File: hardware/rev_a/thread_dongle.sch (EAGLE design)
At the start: 5 parts, among them IC1 CP2102, J1 USB-A-MALE-PLUG

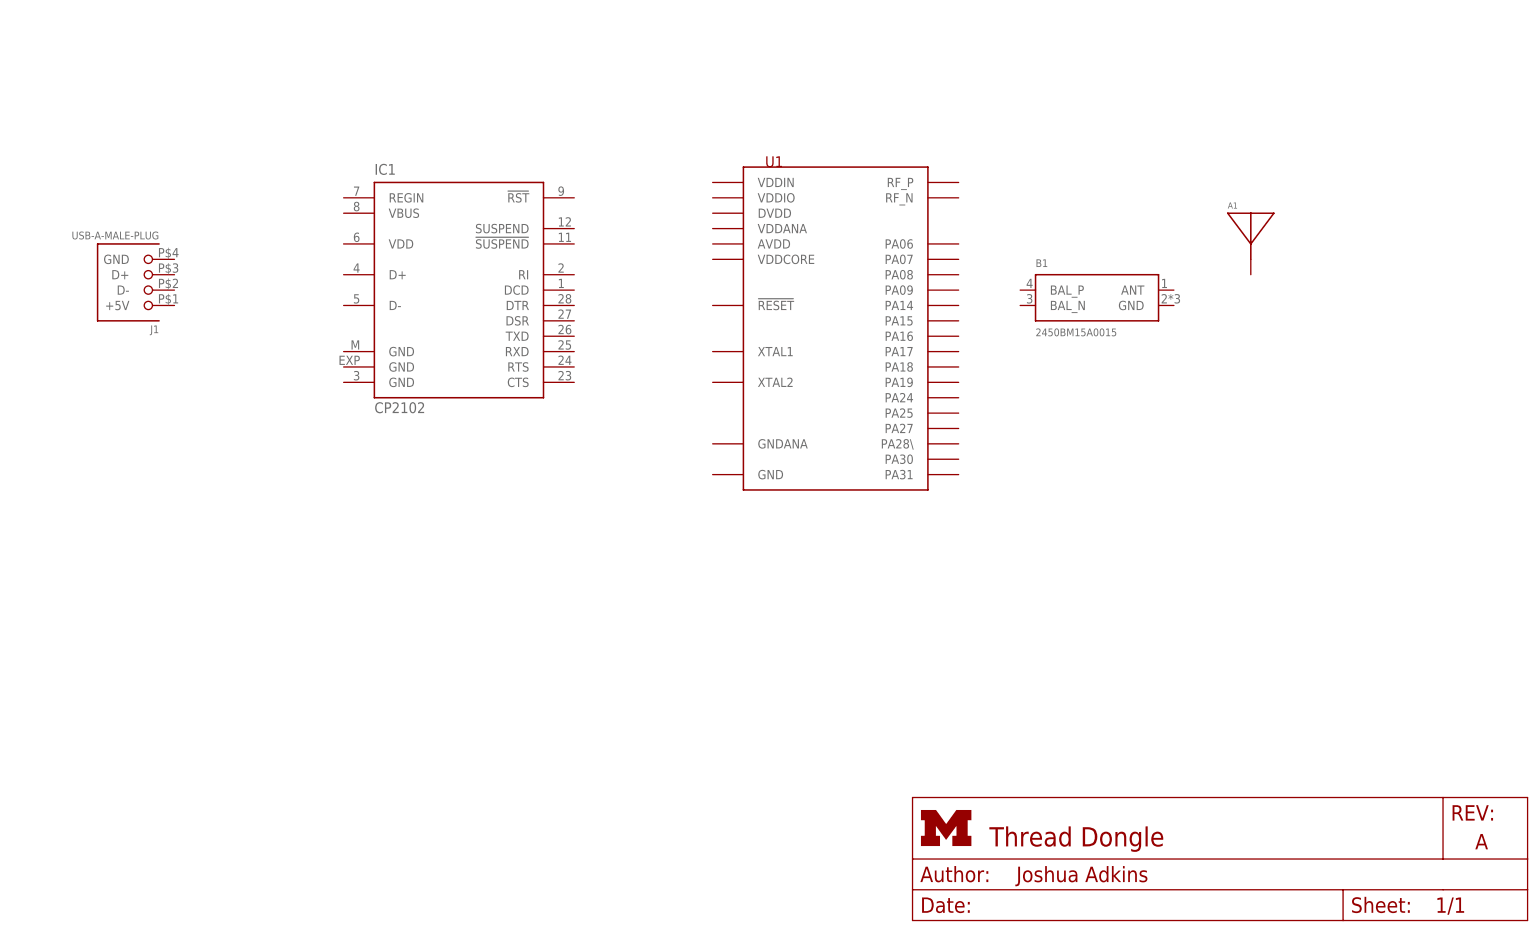
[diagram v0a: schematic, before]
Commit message: added routed board and schematic
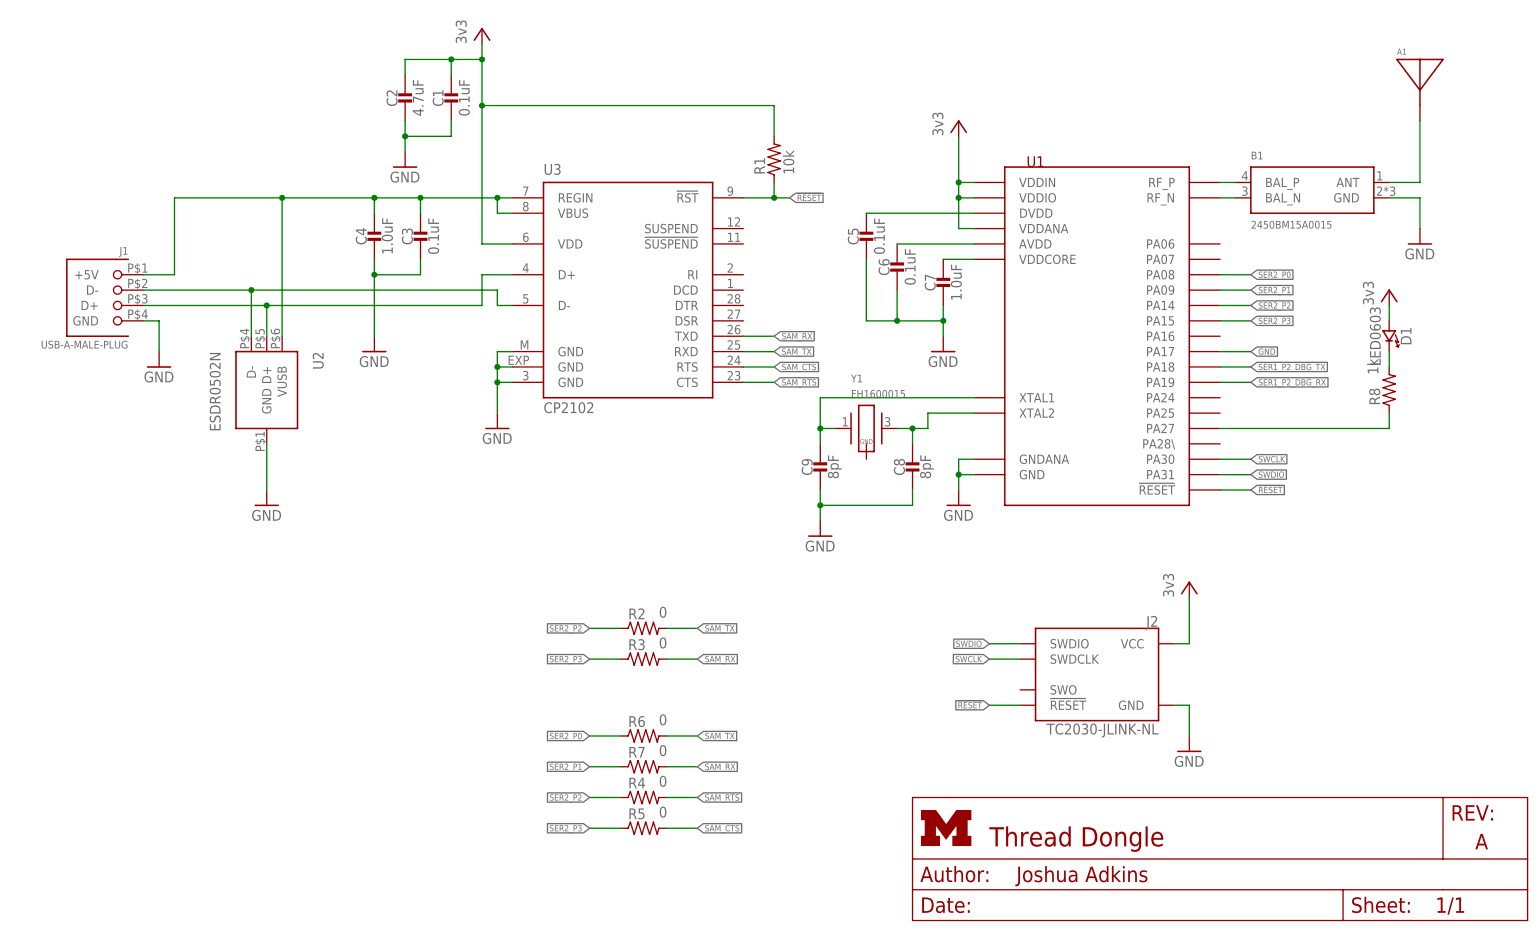
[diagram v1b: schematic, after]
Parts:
- removed IC1: CP2102, silabs:CP2102
- added C1, C3, C5, C6: 0.1uF, passives:CAPACITOR0402_CAP
- added C2: 4.7uF, passives:CAPACITOR0402_CAP
- added C4, C7: 1.0uF, passives:CAPACITOR0402_CAP
- added C8, C9: 8pF, passives:CAPACITOR0402_CAP
- added D1: LED0603, leds:LED0603
- added J2: TC2030-JLINK-NL, connector:TC2030-JLINK-NL
- added R1: 10k, passives:RESISTOR0402_RES
- added R2, R3, R4, R5, R6, R7: 0, passives:RESISTOR0402_RES
- added R8: 1k, passives:RESISTOR0402_RES
- added U2: ESDR0502N, chips:ESDR0502N
- added U3: CP2102, silabs:CP2102
- added Y1: FH1600015, crystals:FH1600015
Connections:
- new net !RESET: J2.!RESET, R1.1, U1.!RESET, U3.!RST
- new net GND: B1.GND, C1.2, C2.2, C3.2, C4.2, C5.2, C6.2, C7.2, C8.2, C9.2, J1.GND, J2.GND, U1.GND, U1.GNDANA, U1.PA17, U2.GND, U3.GND, U3.GND@EXP, U3.GND@M
- new net N$1: B1.BAL_P, U1.RF_P
- new net N$10: C8.1, U1.XTAL2, Y1.2
- new net N$15: C5.1, U1.DVDD
- new net N$16: C6.1, U1.AVDD
- new net N$17: C7.1, U1.VDDCORE
- new net N$2: B1.BAL_N, U1.RF_N
- new net N$3: A1.ANTENNA, B1.ANT
- new net N$4: J1.D-, U2.D-, U3.D-
- new net N$5: J1.D+, U2.D+, U3.D+
- new net N$6: C3.1, C4.1, J1.+5V, U2.VUSB, U3.REGIN, U3.VBUS
- new net N$7: D1.CATHODE, R8.2
- new net N$8: R8.1, U1.PA27
- new net N$9: C9.1, U1.XTAL1, Y1.1
- new net SAM_CTS: R5.2, U3.RTS
- new net SAM_RTS: R4.2, U3.CTS
- new net SAM_RX: R3.2, R7.2, U3.TXD
- new net SAM_TX: R2.2, R6.2, U3.RXD
- new net SER1_P2_DBG_RX: U1.PA19
- new net SER1_P2_DBG_TX: U1.PA18
- new net SER2_P0: R6.1, U1.PA08
- new net SER2_P1: R7.1, U1.PA09
- new net SER2_P2: R2.1, R4.1, U1.PA14
- new net SER2_P3: R3.1, R5.1, U1.PA15
- new net SWCLK: J2.SWDCLK, U1.PA30
- new net SWDIO: J2.SWDIO, U1.PA31
- new net VCC: C1.1, C2.1, D1.ANODE, J2.VCC, R1.2, U1.VDDANA, U1.VDDIN, U1.VDDIO, U3.VDD
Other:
- note added: "OPENTHREAD DEFAULT CONFIGURATION"
- note added: "VALID FLOWCONTROL CONFIGURATION"
- moved on the sheet: A1, B1, J1, U1
